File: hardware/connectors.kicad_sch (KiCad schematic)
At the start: 3 parts, among them J3 PWM1, J5 PWM2, J6 POWER & CAN & SPI2

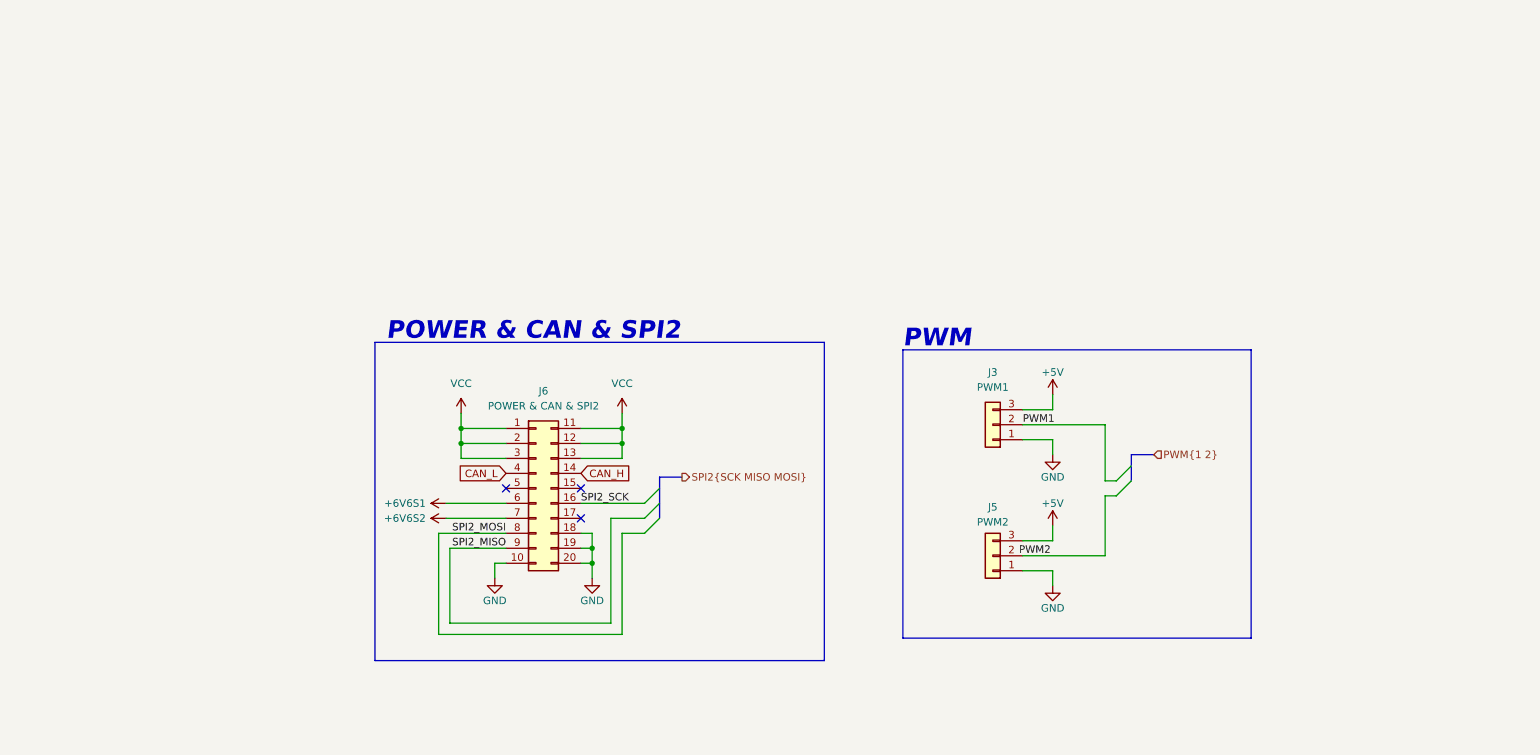
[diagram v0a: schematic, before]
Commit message: Poprawione busy, brak errorow
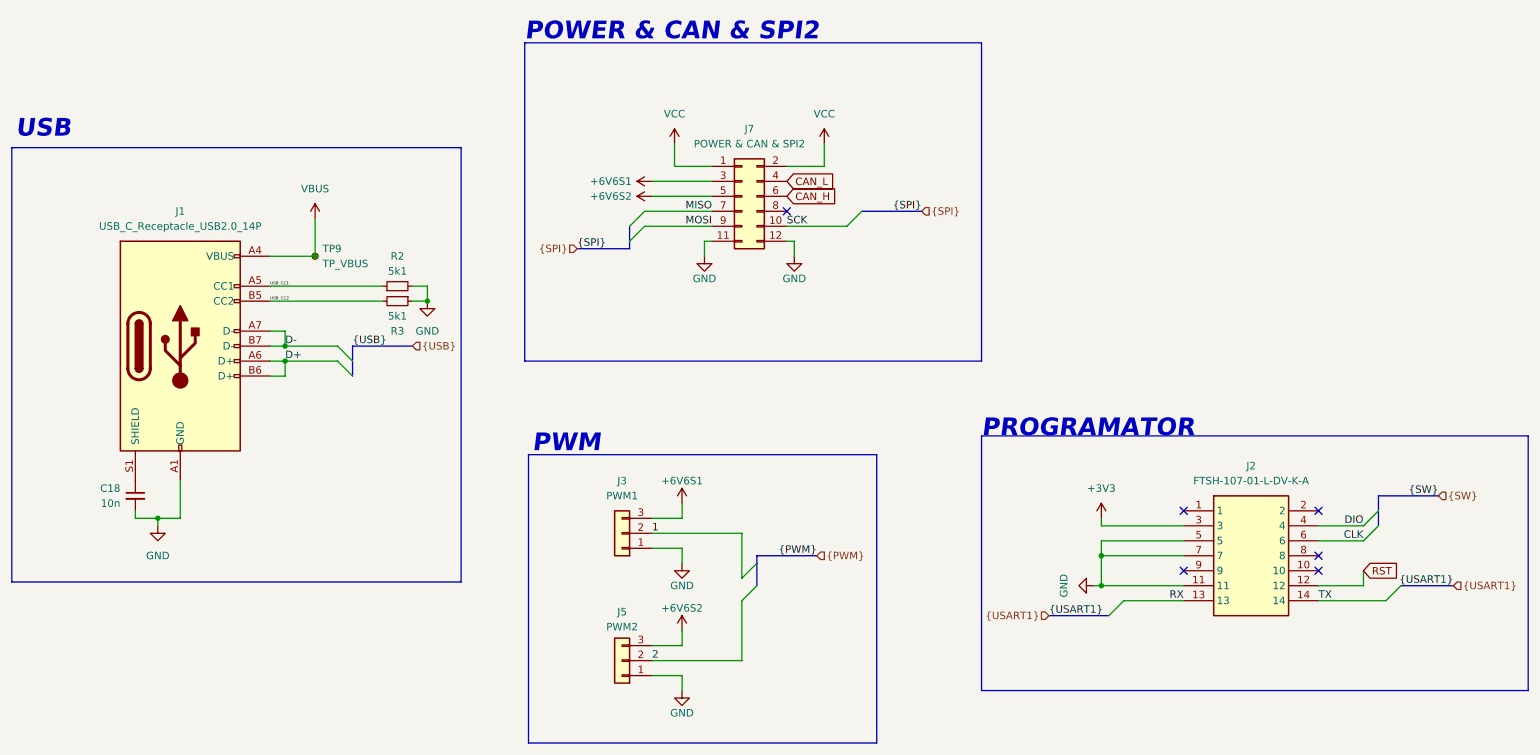
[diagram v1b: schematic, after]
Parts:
- removed J6: POWER & CAN & SPI2, symbol Connector_Generic:Conn_02x10_Top_Bottom
- added C18: 10n, Capacitor_SMD:C_0603_1608Metric_Pad1.08x0.95mm_HandSolder, symbol Device:C_Small
- added J1: USB_C_Receptacle_USB2.0_14P, symbol Connector:USB_C_Receptacle_USB2.0_14P
- added J2: FTSH-107-01-L-DV-K-A, FTSH-107-XX-YYY-DV-K-A, symbol FTSH-107-01-L-DV-K-A:FTSH-107-01-L-DV-K-A
- added J7: POWER & CAN & SPI2, symbol Connector_Generic:Conn_02x06_Odd_Even
- added R2, R3: 5k1, symbol Device:R_Small
- added TP9: TP_VBUS, symbol Connector:TestPoint_Small
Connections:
- net +6V6S1: now also J3.3 (Pin_3), J7.3 (Pin_3)
- net +6V6S2: now also J5.3 (Pin_3), J7.5 (Pin_5)
- net CAN_H: now also J7.6 (Pin_6)
- net CAN_L: now also J7.4 (Pin_4)
- net GND: now also C18.2, J1.A1 (GND), J1.A12 (GND), J1.B1 (GND), J1.B12 (GND), J2.11, J2.5, J2.7, J7.11 (Pin_11), J7.12 (Pin_12), R2.2, R3.1
- net VCC: now also J7.1 (Pin_1), J7.2 (Pin_2)
- net 2: now reaches J5.2 (Pin_2)
- removed net +5V: J3.3 (Pin_3), J5.3 (Pin_3)
- net PWM1 renamed 1
- new net: C18.1, J1.S1 (SHIELD)
- new net +3V3: J2.3
- new net CLK: J2.6
- new net D+: J1.A6 (D+), J1.B6 (D+)
- new net D-: J1.A7 (D-), J1.B7 (D-)
- new net DIO: J2.4
- new net MISO: J7.7 (Pin_7)
- new net MOSI: J7.9 (Pin_9)
- new net RST: J2.12
- new net RX: J2.13
- new net SCK: J7.10 (Pin_10)
- new net TX: J2.14
- new net USB_CC1: J1.A5 (CC1), R2.1
- new net USB_CC2: J1.B5 (CC2), R3.2
- new net VBUS: J1.A4 (VBUS), J1.A9 (VBUS), J1.B4 (VBUS), J1.B9 (VBUS), TP9.1
- no-connect marks 3 -> 6
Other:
- note added: "PROGRAMATOR"
- note added: "USB"
- moved on the sheet: J3, J5
